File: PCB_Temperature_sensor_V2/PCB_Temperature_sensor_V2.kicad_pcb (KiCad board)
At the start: 2 copper layers, 41.1 x 55.2 mm, 16 parts, among them J1 Conn_01x04_Pin, J2 Conn_01x02_Pin, J3 Conn_01x02_Pin, U1 LM35-LP, U2 LM358, U3 LM358

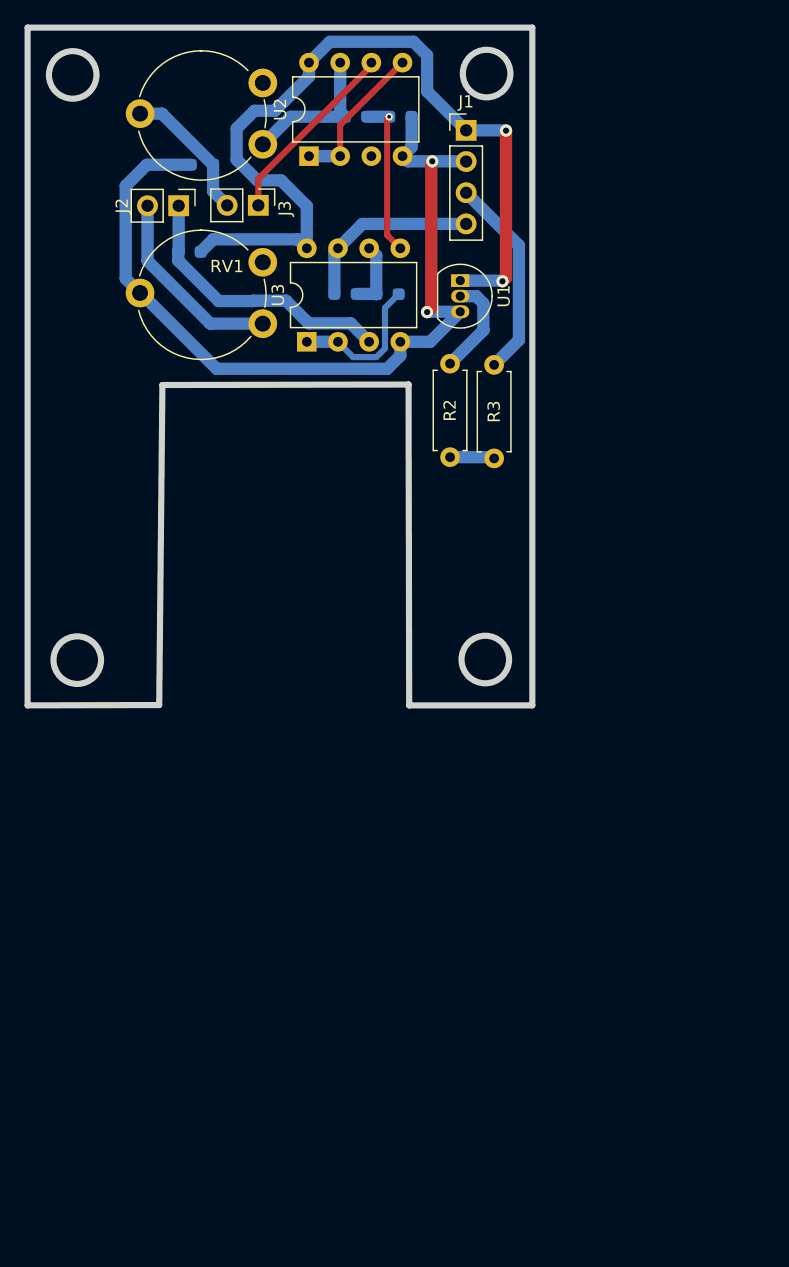
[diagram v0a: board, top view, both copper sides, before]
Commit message: final
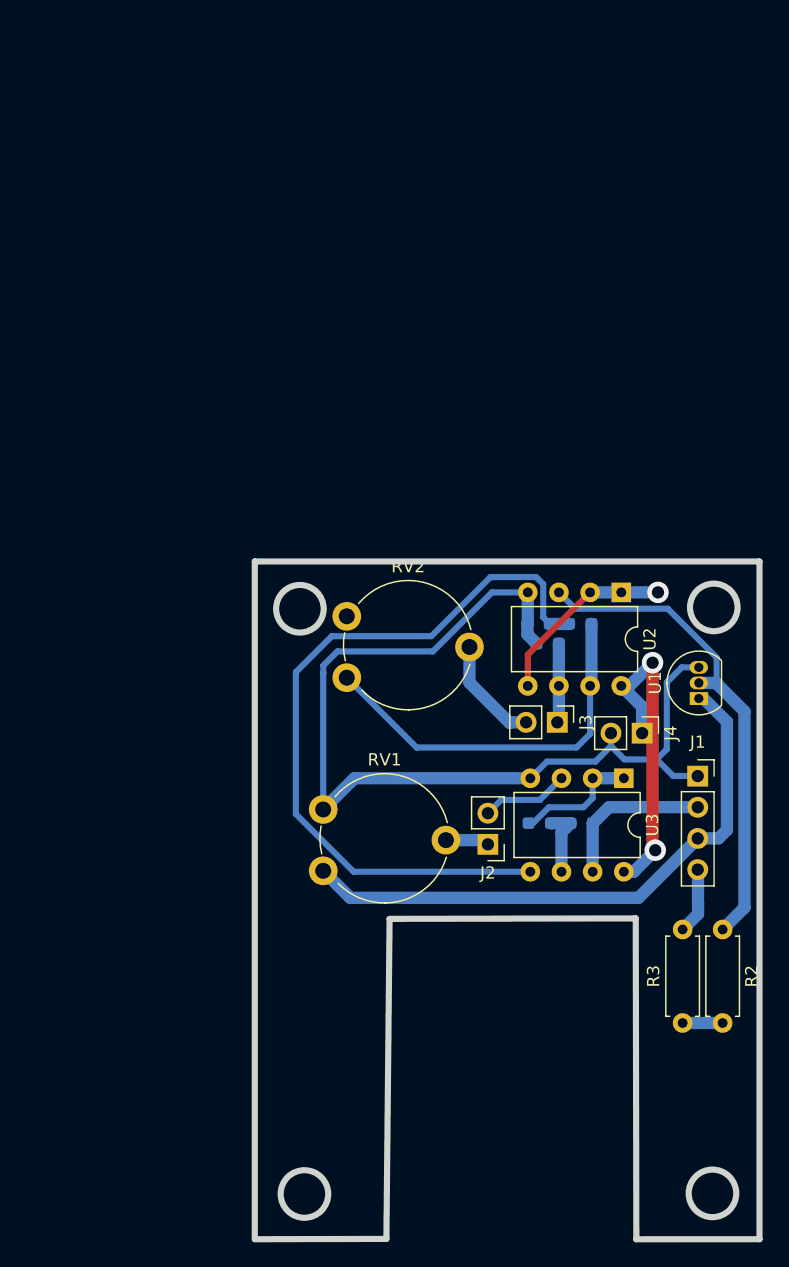
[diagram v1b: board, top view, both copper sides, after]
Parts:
- removed R1: R, Resistor_SMD:R_0603_1608Metric_Pad0.98x0.95mm_HandSolder
- added J4: Conn_01x02_Pin, Connector_PinHeader_2.54mm:PinHeader_1x02_P2.54mm_Vertical, F.Cu at (160.1, 78.1)
- J1: footprint Connector_PinHeader_2.54mm:PinHeader_1x04_P2.54mm_Vertical -> Connector_PinSocket_2.54mm:PinSocket_1x04_P2.54mm_Vertical
- moved J2 57.8 mm to (147.5, 87.1), turned to 180 degrees
- moved J1 55.9 mm to (164.6, 81.6)
- moved R2 51.2 mm to (166.6, 94.1)
- moved RV1 49.8 mm to (134.1, 89.3), turned to 0 degrees
- moved RV2 48.9 mm to (136.0, 73.5), turned to 0 degrees
- moved J3 48.7 mm to (153.1, 77.2)
- moved R3 48.5 mm to (163.4, 101.7)
- moved R4 48.1 mm to (152.4, 70.8)
- moved R8 47.2 mm to (155.1, 85.4), turned to 0 degrees
- moved R5 45.2 mm to (155.0, 69.2), turned to 180 degrees
- moved R7 44.9 mm to (151.7, 85.4), turned to 0 degrees
- moved U3 44.0 mm to (158.6, 81.7), turned to -90 degrees
- moved U2 43.7 mm to (158.4, 66.6), turned to -90 degrees
- moved R6 42.8 mm to (151.6, 69.2), turned to 0 degrees
- moved U1 39.2 mm to (164.7, 75.2), turned to 90 degrees
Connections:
- net Net-(U2A--) renamed V_ADC
- J1 pad 1: 3.3V -> 0
- J1 pad 2: 0 -> V_out
- J1 pad 3: V_3.3 -> 3.3V
- J1 pad 4: V_out -> V_3.3
- R4 pad 2: Net-(J3-Pin_2) -> Net-(J3-Pin_1)
- RV1 pad 1: unconnected-(RV1-Pad1) -> 3.3V
- RV1 pad 2: 0 -> Net-(J2-Pin_1)
- RV1 pad 3: Net-(J2-Pin_2) -> 0
- RV2 pad 1: unconnected-(RV2-Pad1) -> Net-(R5-Pad1)
- RV2 pad 3: Net-(R5-Pad1) -> unconnected-(RV2-Pad3)
- U2 pad 3: V_IN -> Net-(U1-V_{OUT})
- U2 pad 8: 3.3V -> 9V
- U3 pad 3: Net-(J2-Pin_1) -> Net-(J2-Pin_2)
- U3 pad 8: 3.3V -> 9V
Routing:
- net Net-(U3B-+): track 13.0 -> 61.3 mm, vias 1 -> 0
- net Net-(U1-V_{OUT}): track 8.17 -> 40.3 mm
- net 9V: track 0.00 -> 26.6 mm, vias 0 -> 2
- net 3.3V: track 68.7 -> 48.0 mm, vias 2 -> 0
- net Net-(R5-Pad1): track 12.2 -> 31.7 mm
- net Net-(J2-Pin_1): track 22.8 -> 3.56 mm
- net V_3.3: track 16.6 -> 5.42 mm
- net 0: track 70.5 -> 79.8 mm, vias 2 -> 0
- net Net-(J3-Pin_1): track 15.4 -> 6.51 mm
- net Net-(J2-Pin_2): track 16.0 -> 7.22 mm
- net V_ADC: track 12.3 -> 15.3 mm, vias 0 -> 1
- net Net-(J3-Pin_2): track 11.5 -> 8.90 mm
- net V_out: track 15.1 -> 13.1 mm
- net Net-(U3A--): track 12.1 -> 10.2 mm
